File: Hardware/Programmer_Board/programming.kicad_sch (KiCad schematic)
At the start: 19 parts, among them J101 IDC Connector, J102 PicoBlade, J103 USB_C_USB2.0, U1 TPD4E02B04, U102 TPS7A20L_3V3, U103 USBLC6-2SC6

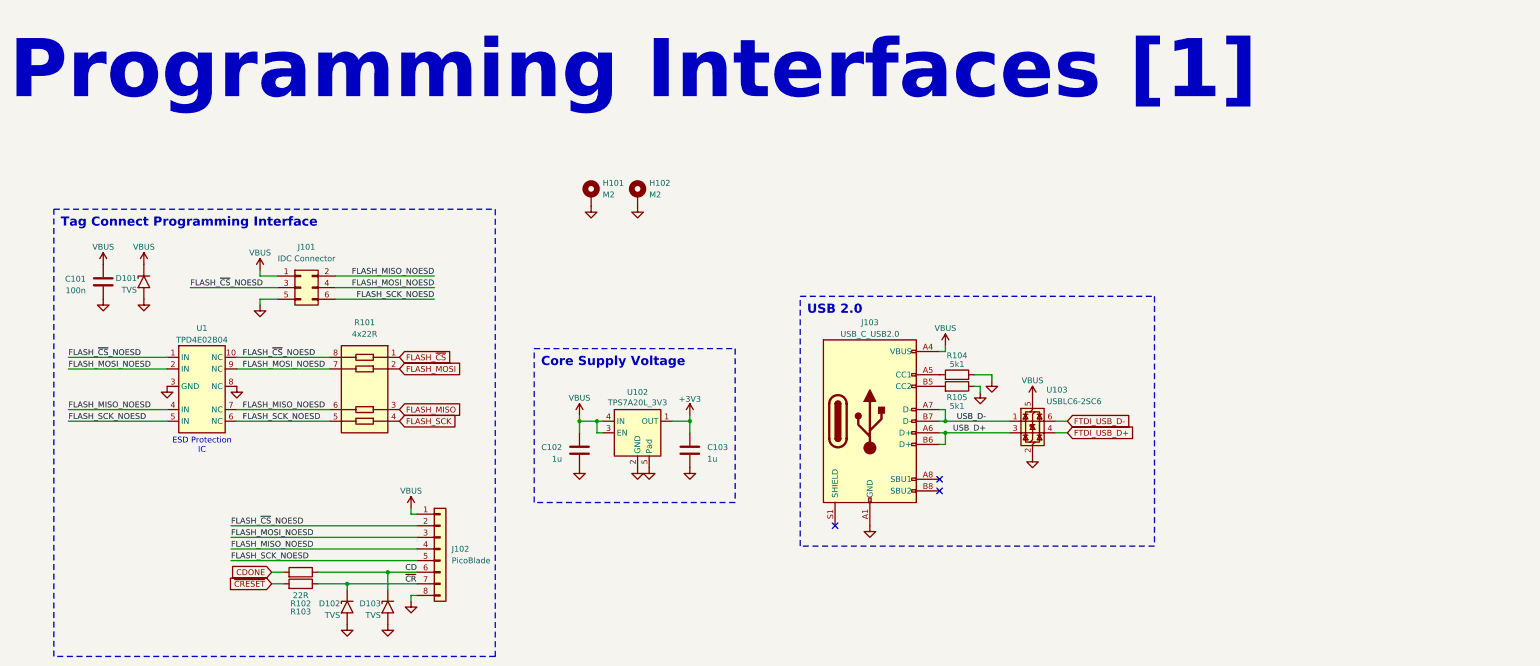
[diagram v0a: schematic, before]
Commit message: Finished design of both programmer and sensor board PCBs
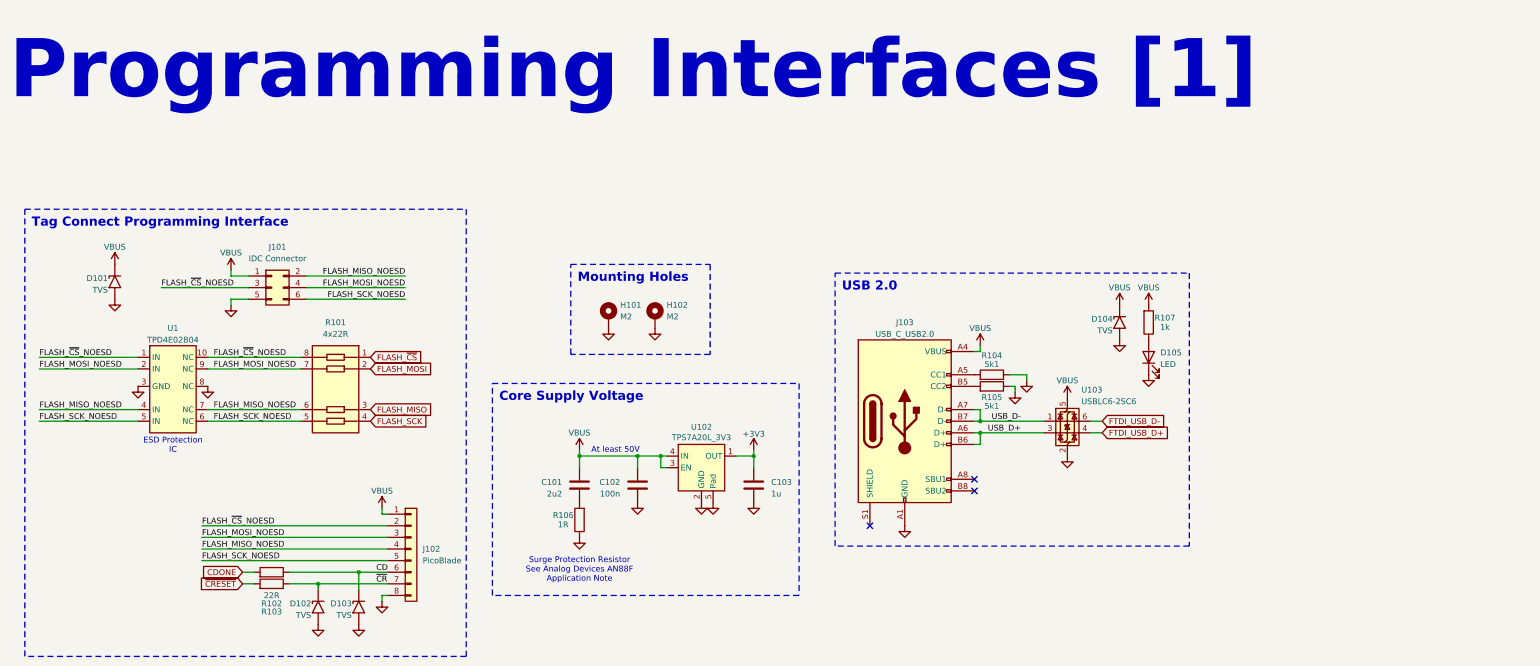
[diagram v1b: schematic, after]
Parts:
- removed C102: 1u, Capacitor_SMD:C_0402_1005Metric, symbol Device:C
- added C101: 2u2, Capacitor_SMD:C_0603_1608Metric, symbol Device:C
- added D104: TVS, Diode_SMD:D_0402_1005Metric, symbol Diode:1.5KExxA
- added D105: LED, LED_SMD:LED_0603_1608Metric, symbol Device:LED
- added R106: 1R, Resistor_SMD:R_0402_1005Metric, symbol Device:R
- added R107: 1k, Resistor_SMD:R_0402_1005Metric, symbol Device:R
- J101: Distributor Link 2 (none) -> https://www.mouser.sk/ProductDetail/Samtec/TST-103-05-L-D-R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
- renumbered C101 to C102
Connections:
- net GND: now also D104.2 (A2), D105.1 (K), R106.1
- net VBUS: now also C101.1, D104.1 (A1), R107.2
- new net: D105.2 (A), R107.1
- new net: C101.2, R106.2
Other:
- note added: "At least 50V"
- note added: "Surge Protection Resistor See Analog Devices AN88F Application Note"
- moved on the sheet: C102, C103, D101, D102, D103, H101, H102, J101, J102, J103, R101, R102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

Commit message: Finished final PCB checks before manufacturing and uploaded the fabrication files
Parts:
- U1: footprint Package_SON:USON-10_2.5x1.0mm_P0.5mm -> Custom_VoxLink_Footprints:USON-10_2.5x1.0mm_P0.5mm__Reduced_Paste
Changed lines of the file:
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@@
 			)
 		)
-		(property "Footprint" "Package_SON:USON-10_2.5x1.0mm_P0.5mm"
+		(property "Footprint" "Custom_VoxLink_Footprints:USON-10_2.5x1.0mm_P0.5mm__Reduced_Paste"
 			(at 53.34 96.52 0)
 			(effects
@@
 			)
 		)
-		(property "Datasheet" "https://eu.mouser.com/ProductDetail/71-CRCW0402-5.1K-E3"
+		(property "Datasheet" "https://eu.mouser.com/ProductDetail/71-CRCW040222R0JNEDC"
 			(at 74.93 137.16 0)
 			(effects
@@
 			)
 		)
-		(property "Datasheet" "https://eu.mouser.com/ProductDetail/71-CRCW0402-5.1K-E3"
+		(property "Datasheet" "https://eu.mouser.com/ProductDetail/71-CRCW040222R0JNEDC"
 			(at 74.93 139.7 0)
 			(effects
@@
 			)
 		)
-		(property "Datasheet" "https://www.mouser.sk/ProductDetail/Vishay-Dale/RCC06031R00FKEA?qs=GedFDFLaBXHoNHSIHYHq8Q%3D%3D"
+		(property "Datasheet" "https://www.mouser.sk/ProductDetail/Vishay-Draloric/RCS04021R00JNED?qs=NKmfXavxMayJEsE2Q0i2Jg%3D%3D"
 			(at 142.24 125.73 0)
 			(effects
@@
 			)
 		)
-		(property "Datasheet" "https://eu.mouser.com/ProductDetail/Panasonic/EXB-38V220JV?qs=uA7cY%2Fh6FfWz7RTZfU3o3w%3D%3D&srsltid=AfmBOopzjZsMxnOYcXJV453D_R8g91dh9OwbKtkf1b7QjBlPLoZ2zN1B"
+		(property "Datasheet" "https://eu.mouser.com/ProductDetail/Panasonic/EXB-N8V220JX?qs=bx0%2FPCyAc7556mtSQRzOoA%3D%3D"
 			(at 88.9 96.52 0)
 			(effects
